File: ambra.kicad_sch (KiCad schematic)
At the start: 27 parts, among them J3 MTSW-103-07-S-S-225, J4 MTSW-103-07-S-S-225, J5 MJ-4PP-9, J6 B2B-ZR_LF__SN_, SW1 SW_SPDT, U1 ProMicro_r

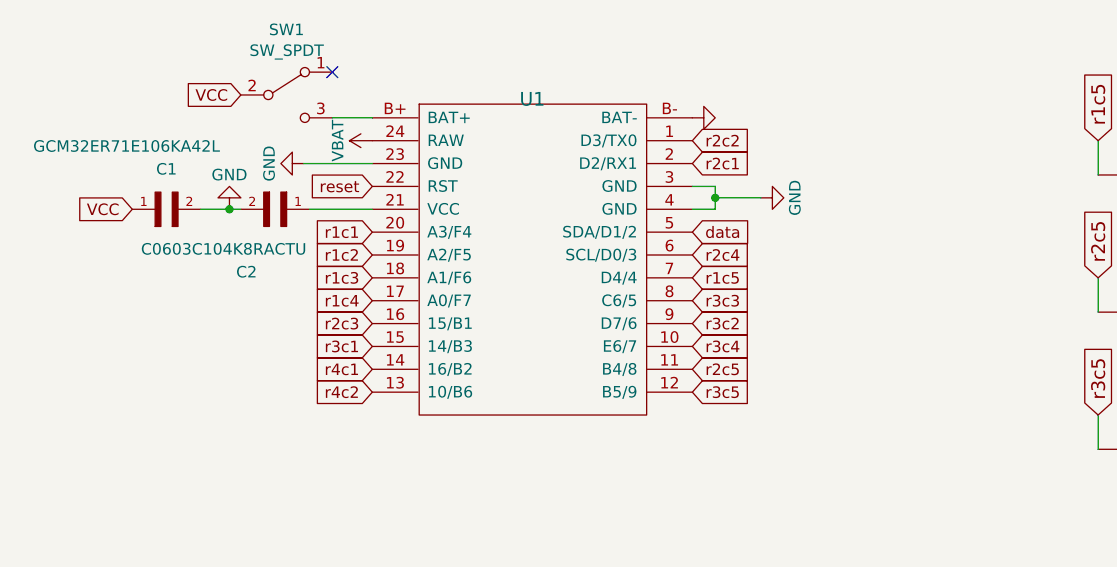
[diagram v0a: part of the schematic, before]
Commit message: Add files via upload
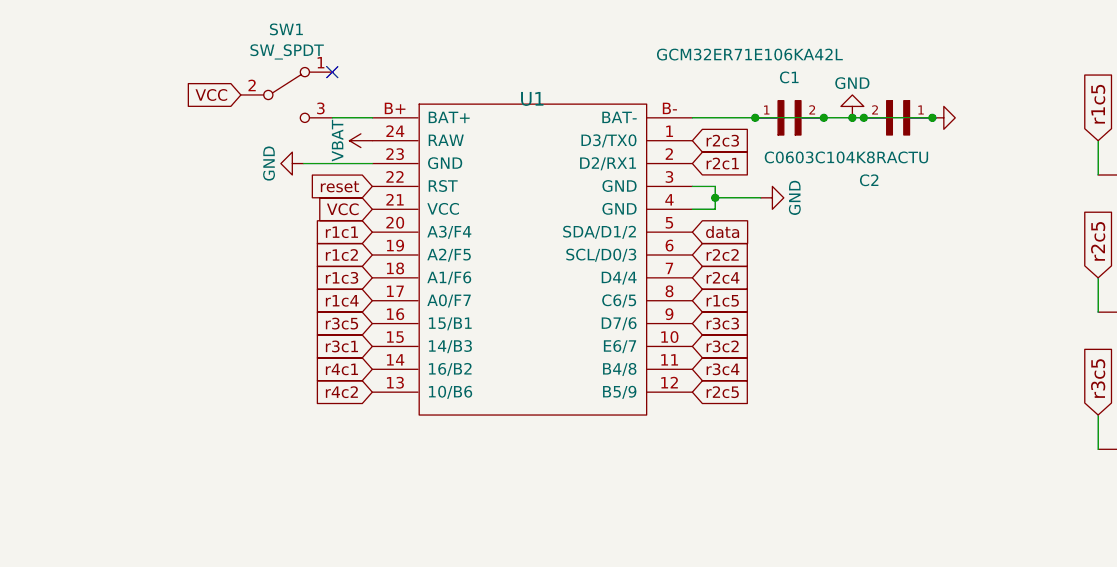
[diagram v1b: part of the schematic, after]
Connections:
- net GND: now also C1.1, C2.1
- net VCC: now also U1.21 (VCC); no longer C1.1
- net r1c5: now also U1.8 (C6/5); no longer U1.7 (D4/4)
- net r2c2: now also U1.6 (SCL/D0/3); no longer U1.1 (D3/TX0)
- net r2c3: now also U1.1 (D3/TX0); no longer U1.16 (15/B1)
- net r2c4: now also U1.7 (D4/4); no longer U1.6 (SCL/D0/3)
- net r2c5: now also U1.12 (B5/9); no longer U1.11 (B4/8)
- net r3c2: now also U1.10 (E6/7); no longer U1.9 (D7/6)
- net r3c3: now also U1.9 (D7/6); no longer U1.8 (C6/5)
- net r3c4: now also U1.11 (B4/8); no longer U1.10 (E6/7)
- net r3c5: now also U1.16 (15/B1); no longer U1.12 (B5/9)
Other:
- moved on the sheet: C1, C2

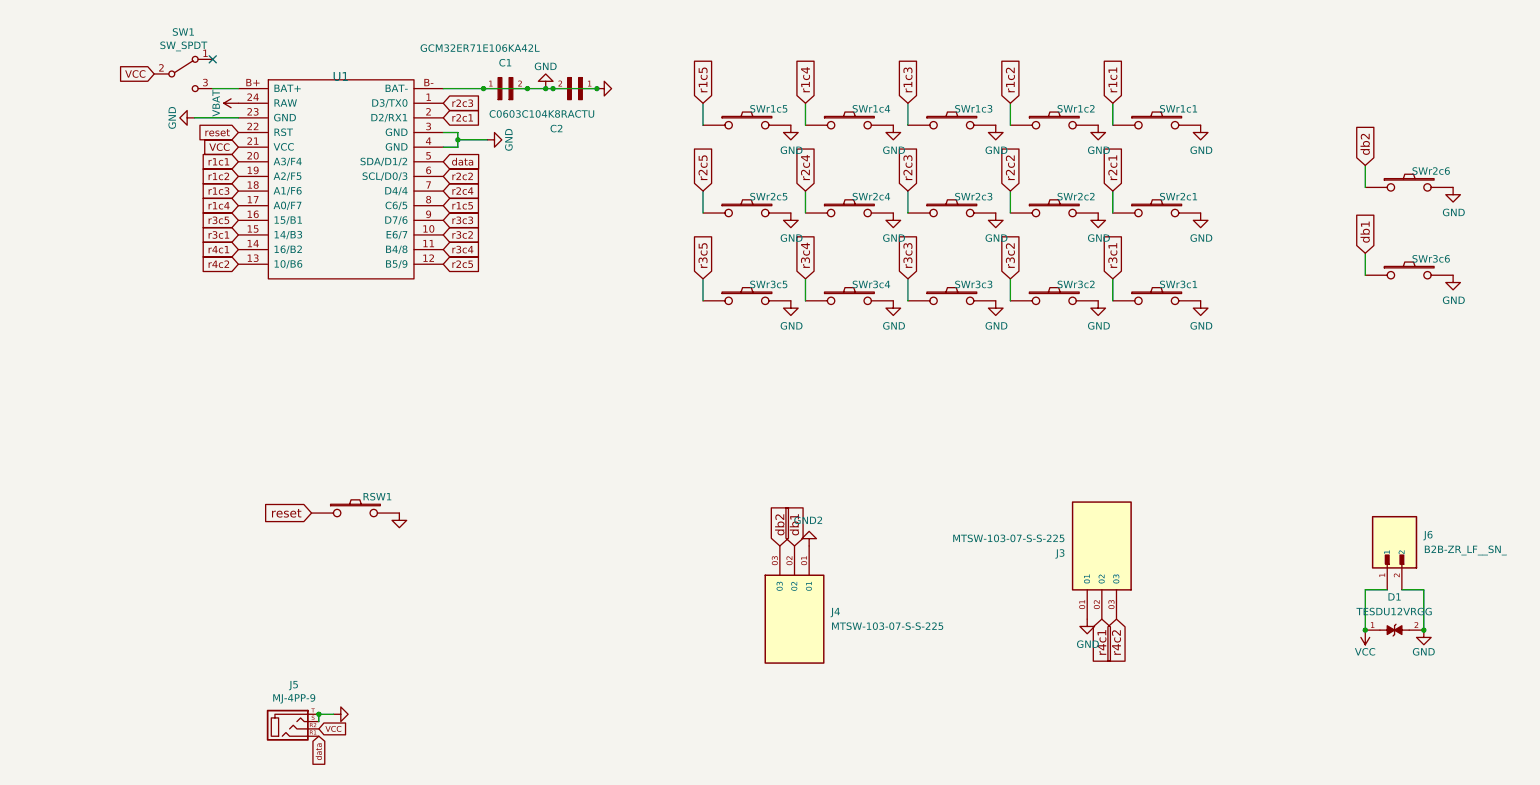
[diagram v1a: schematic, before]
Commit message: Add files via upload
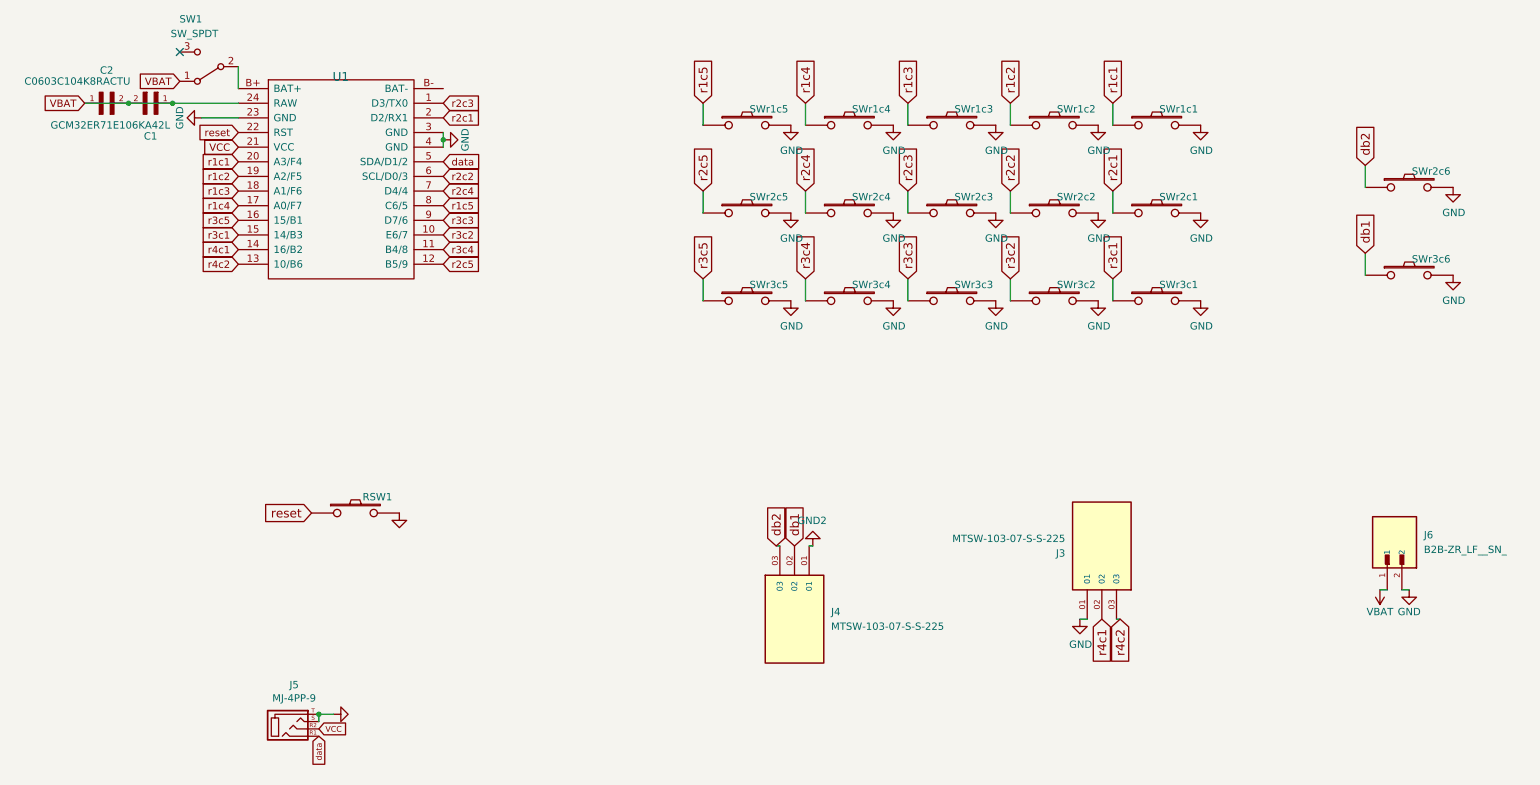
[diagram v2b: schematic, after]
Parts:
- removed D1: TESDU12VRGG, my syms-foots:TVS-P6SMBJ5.0CA, symbol TESDU12VRGG:TESDU12VRGG
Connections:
- net GND: no longer C1.1, C1.2, C2.1, C2.2, U1.B- (BAT-)
- net VBAT: now also C1.1, C1.2, C2.1, C2.2, J6.1, SW1.1 (A)
- net VCC: no longer J6.1, SW1.2 (B)
- net at U1.B+ (BAT+): now also SW1.2 (B); no longer SW1.3 (C)
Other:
- moved on the sheet: C1, C2, SW1
